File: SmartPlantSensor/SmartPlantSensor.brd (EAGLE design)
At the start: 25 x 100 mm, 13 parts

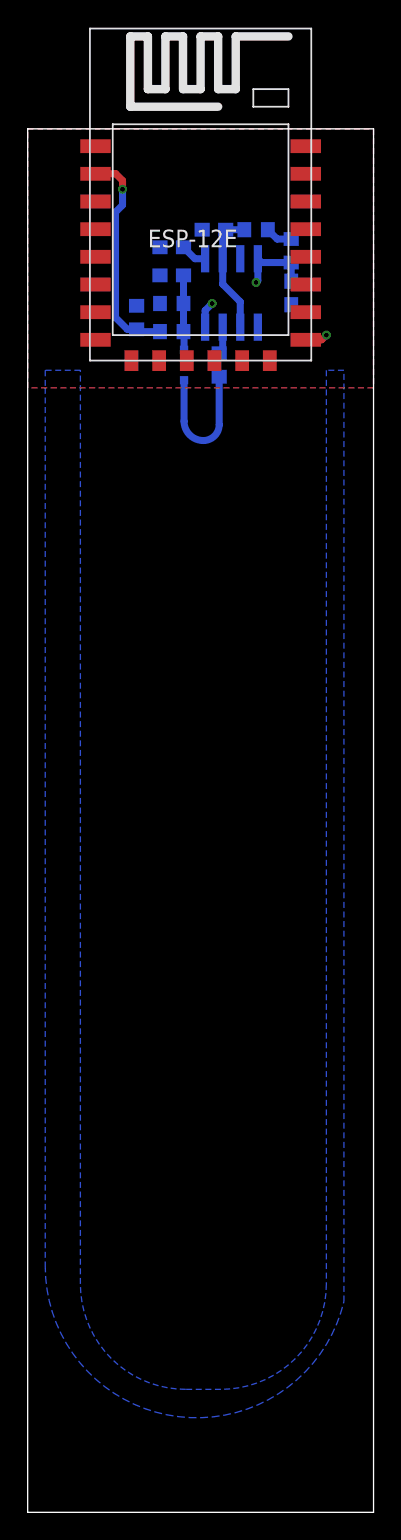
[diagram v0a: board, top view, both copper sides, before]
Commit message: Release v1.0.0
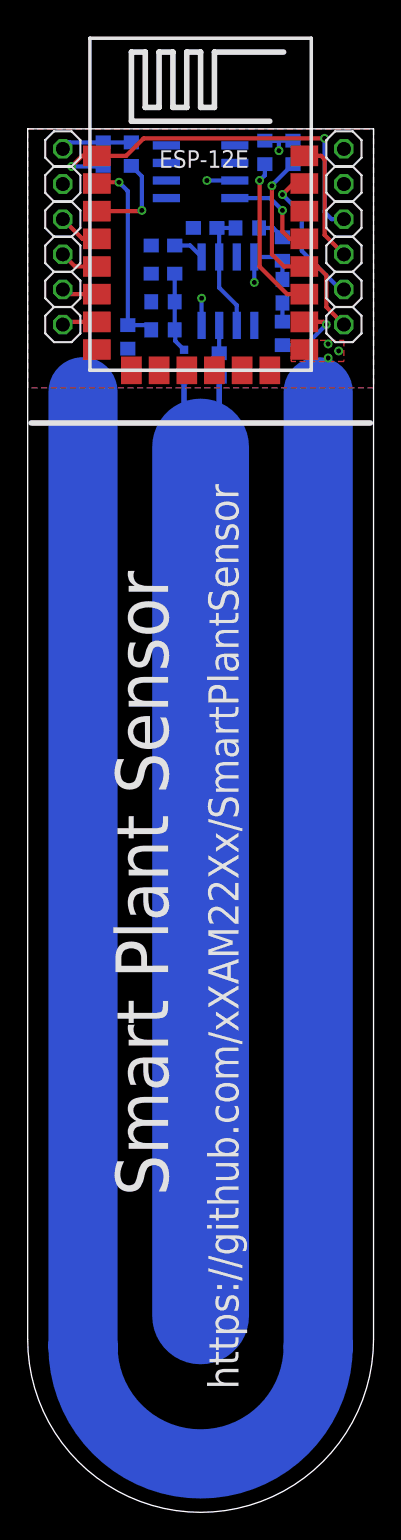
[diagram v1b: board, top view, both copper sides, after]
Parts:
- removed C5: 10nF, rcl:C0603
- removed U$1: TLC555CDR, HeRo:SOIC127P600X175-8
- removed U$2: ESP-12E, HeRo:ESP-12E
- added C1: 10nF, rcl:C0603
- added DS18B20: DS18B20Z+, MaximIntegrated:SOIC8
- added ESP-12E: ESP-12E, ESP:ESP-12E
- added JP10, JP11, JP12, JP13, JP14, JP3, JP4, JP5, JP6, JP7, JP8, JP9: (no value), pinhead:1X01
- added R10, R11, R7, R8, R9: 10k, rcl:R0603
- added TLC555: TLC555CD, TexasInstruments:SOIC8
- moved R6 1.53 mm to (7.24, 85.0), turned to 90 degrees
- moved R4 0.65 mm to (15.9, 92.8)
- moved C4 0.65 mm to (12.8, 92.8)
- moved R1 0.65 mm to (9.78, 85.5)
- moved C3 0.65 mm to (18.4, 88.3)
- moved R5 0.65 mm to (18.4, 91.3)
- moved C2 0.65 mm to (9.78, 89.5)
- moved R2 0.65 mm to (9.78, 87.5)
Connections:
- removed net N$7: C5.2, U$1.5
- new net 1WIRE: DS18B20.4, ESP-12E.19
- new net EN: ESP-12E.3, R7.1
- new net IO0: ESP-12E.18, JP6.1, R9.1
- new net IO12: ESP-12E.6, JP12.1
- new net IO13: ESP-12E.7, JP11.1
- new net IO14: ESP-12E.5, JP13.1
- new net IO15: ESP-12E.16, R8.2
- new net IO16: ESP-12E.4, JP14.1
- new net IO2: ESP-12E.17, R11.1
- new net N$1: C1.2, TLC555.5
- new net RST: ESP-12E.1, JP5.1, R10.1
- new net RXD: ESP-12E.21, JP8.1
- new net TXD: ESP-12E.22, JP7.1
- net +3V3: now also DS18B20.3, ESP-12E.8, JP3.1, JP9.1, R10.2, R11.2, R7.2, R9.2, TLC555.4, TLC555.8; no longer U$1.4, U$1.8, U$2.VCC
- net ADC: now also ESP-12E.2; no longer U$2.ADC
- net DISH: now also TLC555.7; no longer U$1.7
- net GND: now also C1.1, DS18B20.5, ESP-12E.15, JP10.1, JP4.1, R8.1, TLC555.1; no longer C5.1, U$1.1, U$2.GND
- net OUT: now also TLC555.3; no longer U$1.3
- net T: now also TLC555.2, TLC555.6; no longer U$1.2, U$1.6
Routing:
- net GND: track 1.63 -> 159.1 mm, vias 1 -> 3
- net SENSOR: track 10.0 -> 73.8 mm
- net RST: track 0.00 -> 28.4 mm, vias 0 -> 2
- net IO0: track 0.00 -> 15.8 mm, vias 0 -> 1
- net IO2: track 0.00 -> 11.6 mm, vias 0 -> 1
- net RXD: track 0.00 -> 10.8 mm, vias 0 -> 1
- net +3V3: track 7.56 -> 17.6 mm, vias 2 -> 4
- net TXD: track 0.00 -> 9.01 mm
- net 1WIRE: track 0.00 -> 7.14 mm, vias 0 -> 1
- net EN: track 0.00 -> 6.81 mm, vias 0 -> 1
- net IO15: track 0.00 -> 5.46 mm, vias 0 -> 1
- net IO16: track 0.00 -> 3.05 mm
- net IO14: track 0.00 -> 2.83 mm
- net IO12: track 0.00 -> 2.60 mm
- net IO13: track 0.00 -> 2.54 mm
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- added copper zone on layer 1, net GND
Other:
- outline, holes or cut-outs redrawn
- board text added: "Smart Plant Sensor"
- board text added: "https://github.com/xXAM22Xx/SmartPlantSensor"
